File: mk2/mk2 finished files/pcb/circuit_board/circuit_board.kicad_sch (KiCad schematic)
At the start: 29 parts, among them J1 1x2 Header, J2 1x2 Header, Q1 IRLZ44N, SW1 Momentary

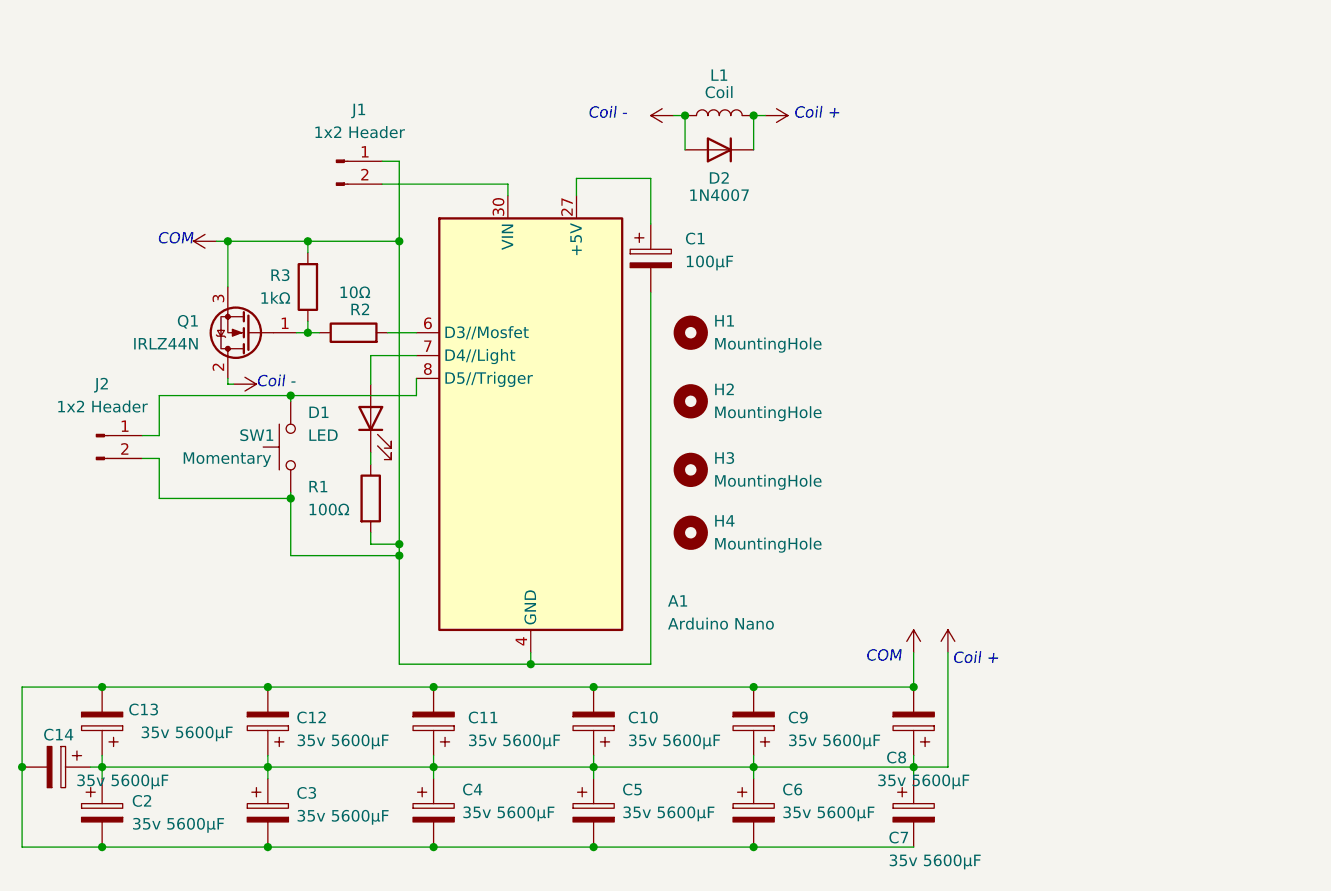
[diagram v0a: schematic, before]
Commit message: PCB Updates
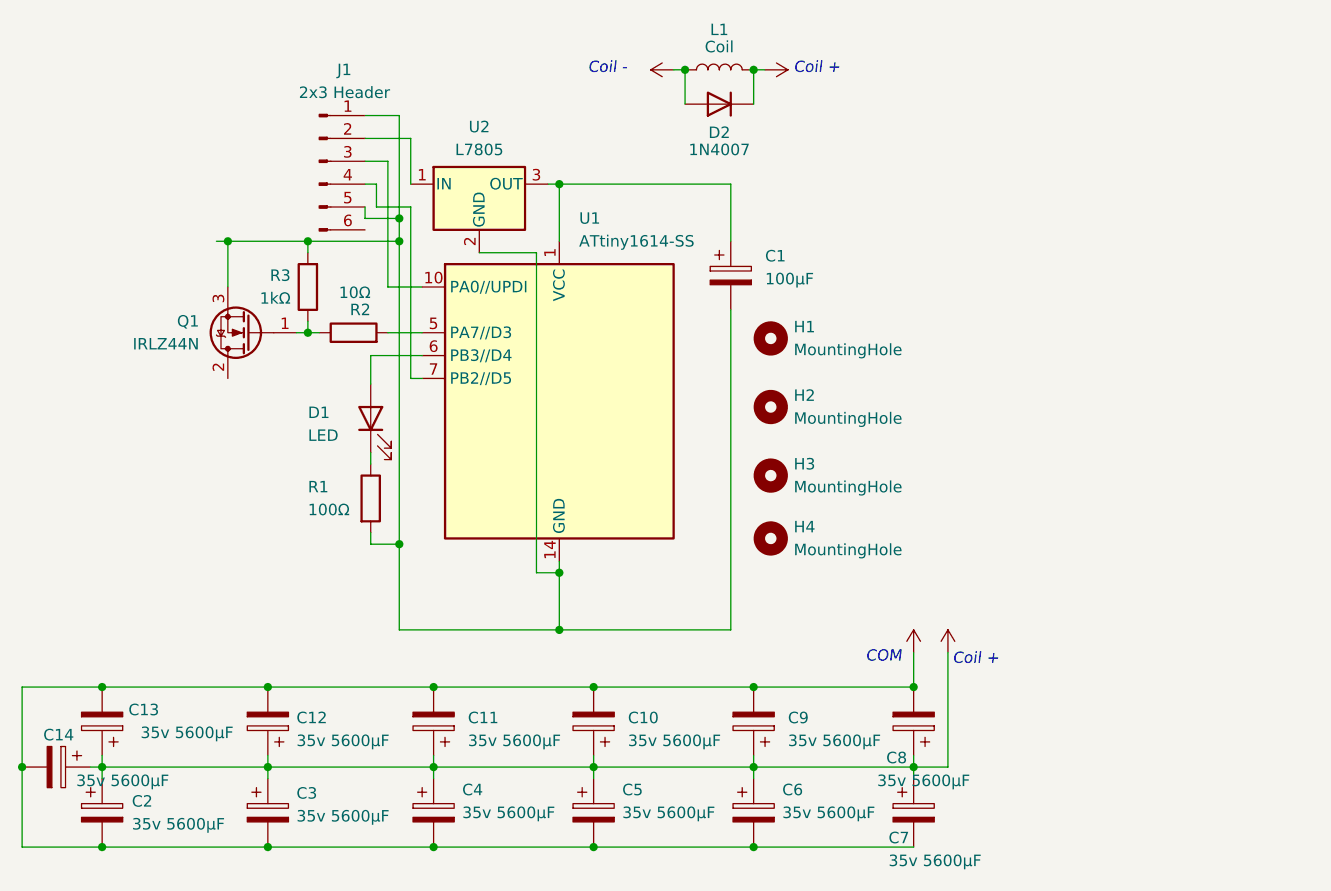
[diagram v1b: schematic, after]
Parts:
- removed A1: Arduino Nano, Module:Arduino_Nano, symbol MCU_Module:Arduino_Nano_Every
- removed J2: 1x2 Header, Connector_PinHeader_2.54mm:PinHeader_1x02_P2.54mm_Horizontal, symbol Connector:Conn_01x02_Male
- removed SW1: Momentary, Button_Switch_THT:SW_PUSH-12mm, symbol Switch:SW_Push
- added U1: ATtiny1614-SS, Package_SO:SOIC-14_3.9x8.7mm_P1.27mm, symbol MCU_Microchip_ATtiny:ATtiny1614-SS
- added U2: L7805, Package_TO_SOT_THT:TO-220-3_Vertical, symbol Regulator_Linear:L7805
- J1: value 1x2 Header -> 2x3 Header; footprint Connector_PinHeader_2.54mm:PinHeader_1x02_P2.54mm_Horizontal -> Connector_PinHeader_2.54mm:PinHeader_1x06_P2.54mm_Vertical_SMD_Pin1Right; symbol Connector:Conn_01x02_Male -> Connector:Conn_01x06_Pin
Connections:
- net +28V: no longer C1.2, J1.1 (Pin_1), Q1.2 (D), Q1.3 (S), R1.2, R3.2
- net at D1.2 (A): now also U1.6 (PB3//D4)
- net at C1.1: now also U1.1 (VCC), U2.3 (OUT)
- net at R2.2: now also U1.5 (PA7//D3)
- net at J1.2 (Pin_2): now also U2.1 (IN)
- new net: C1.2, J1.1 (Pin_1), J1.5 (Pin_5), Q1.3 (S), R1.2, R3.2, U1.14 (GND), U2.2 (GND)
- new net: J1.3 (Pin_3), U1.10 (PA0//UPDI)
- new net: J1.4 (Pin_4), U1.7 (PB2//D5)
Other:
- moved on the sheet: C1, D2, H1, H2, H3, H4, L1

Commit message: Circuit Board Edits
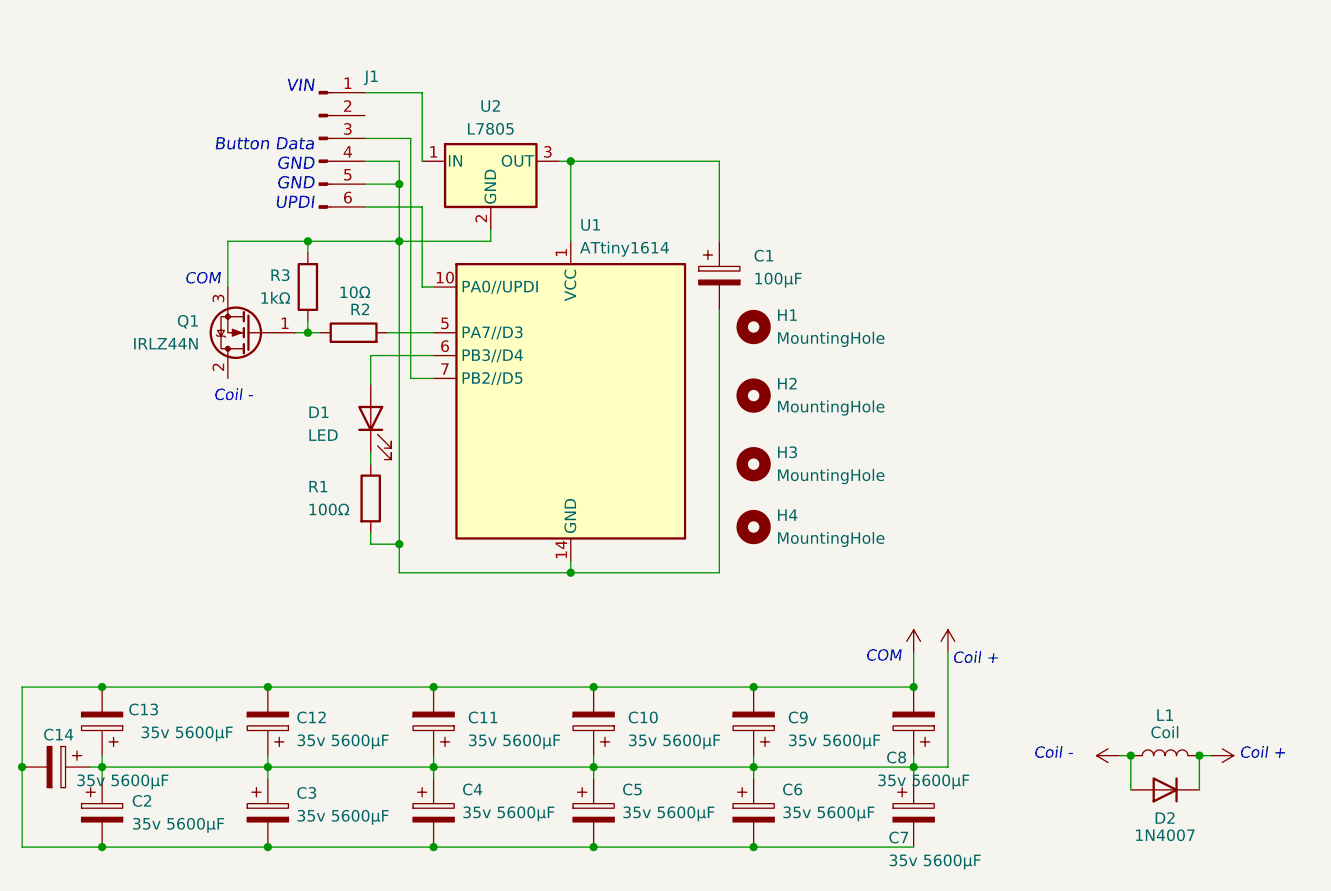
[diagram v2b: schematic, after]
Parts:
- J1: footprint Connector_PinHeader_2.54mm:PinHeader_1x06_P2.54mm_Vertical_SMD_Pin1Right -> Connector_PinHeader_2.54mm:PinHeader_1x06_P2.54mm_Vertical
- U1: value ATtiny1614-SS -> ATtiny1614
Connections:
- net at C1.2, J1.5 (Pin_5), Q1.3 (S)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: now also J1.4 (Pin_4); no longer J1.1 (Pin_1)
- net at U1.10 (PA0//UPDI): now also J1.6 (Pin_6); no longer J1.3 (Pin_3)
- net at U1.7 (PB2//D5): now also J1.3 (Pin_3); no longer J1.4 (Pin_4)
- net at U2.1 (IN): now also J1.1 (Pin_1); no longer J1.2 (Pin_2)
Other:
- note added: "VIN Button Data GND GND UPDI"
- moved on the sheet: C1, D2, H1, H2, H3, H4, J1, L1, U1, U2
